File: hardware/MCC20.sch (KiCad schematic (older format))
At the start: 6 parts, among them J101 Conn_01x20, J102 Conn_01x20

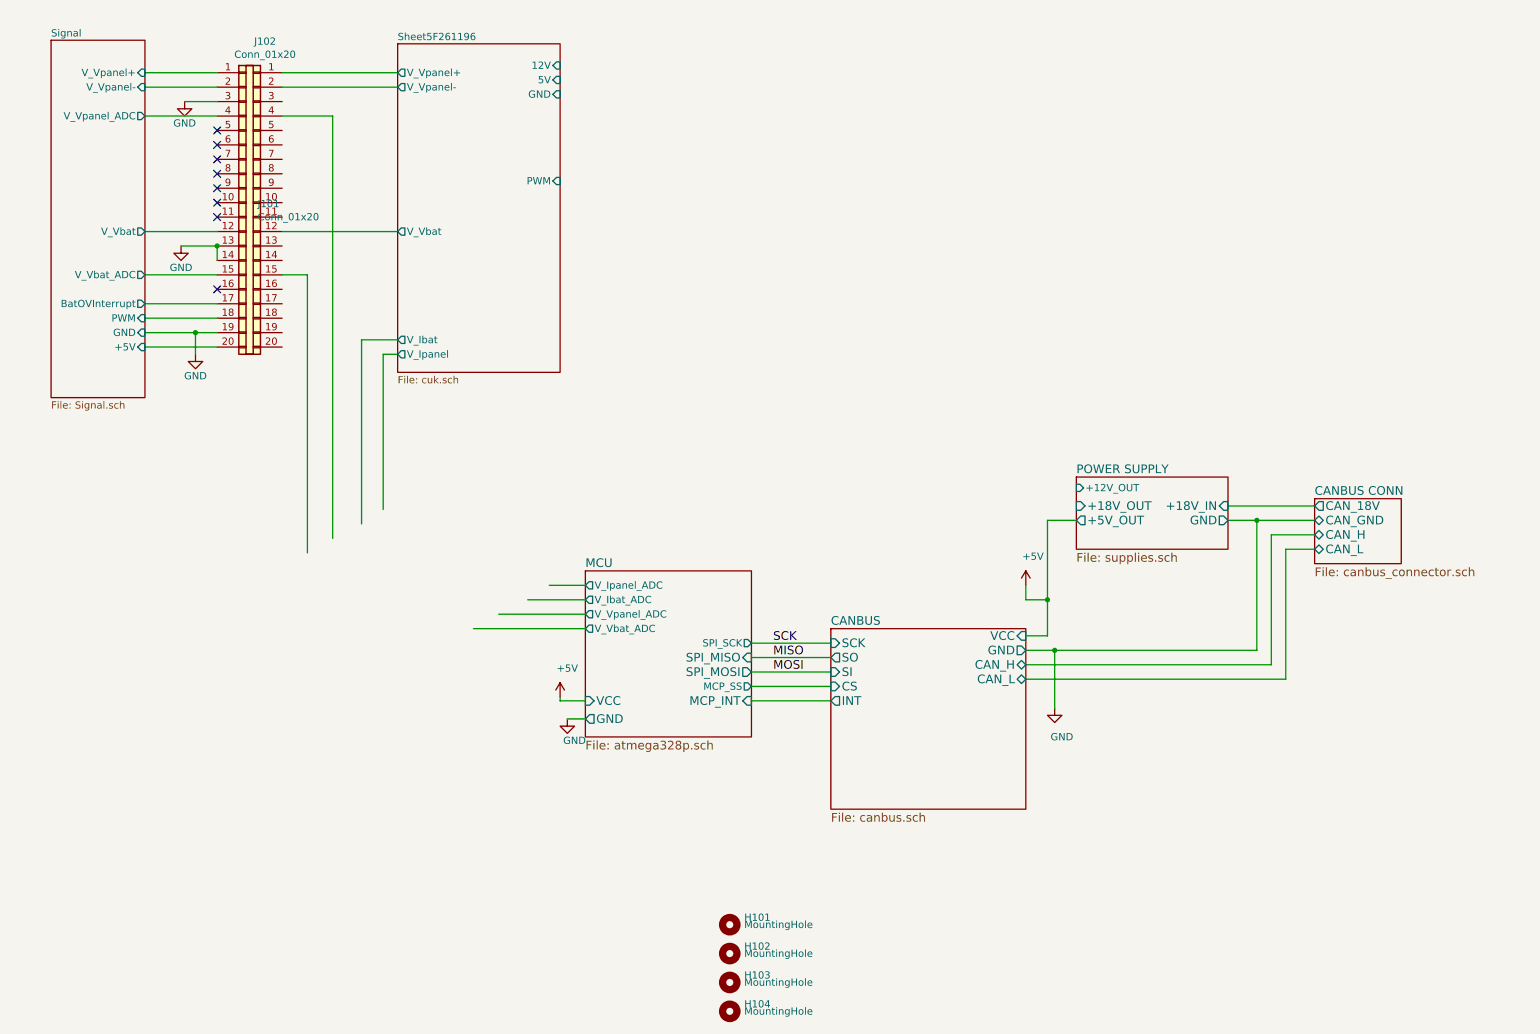
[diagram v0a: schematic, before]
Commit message: schematic and footprint
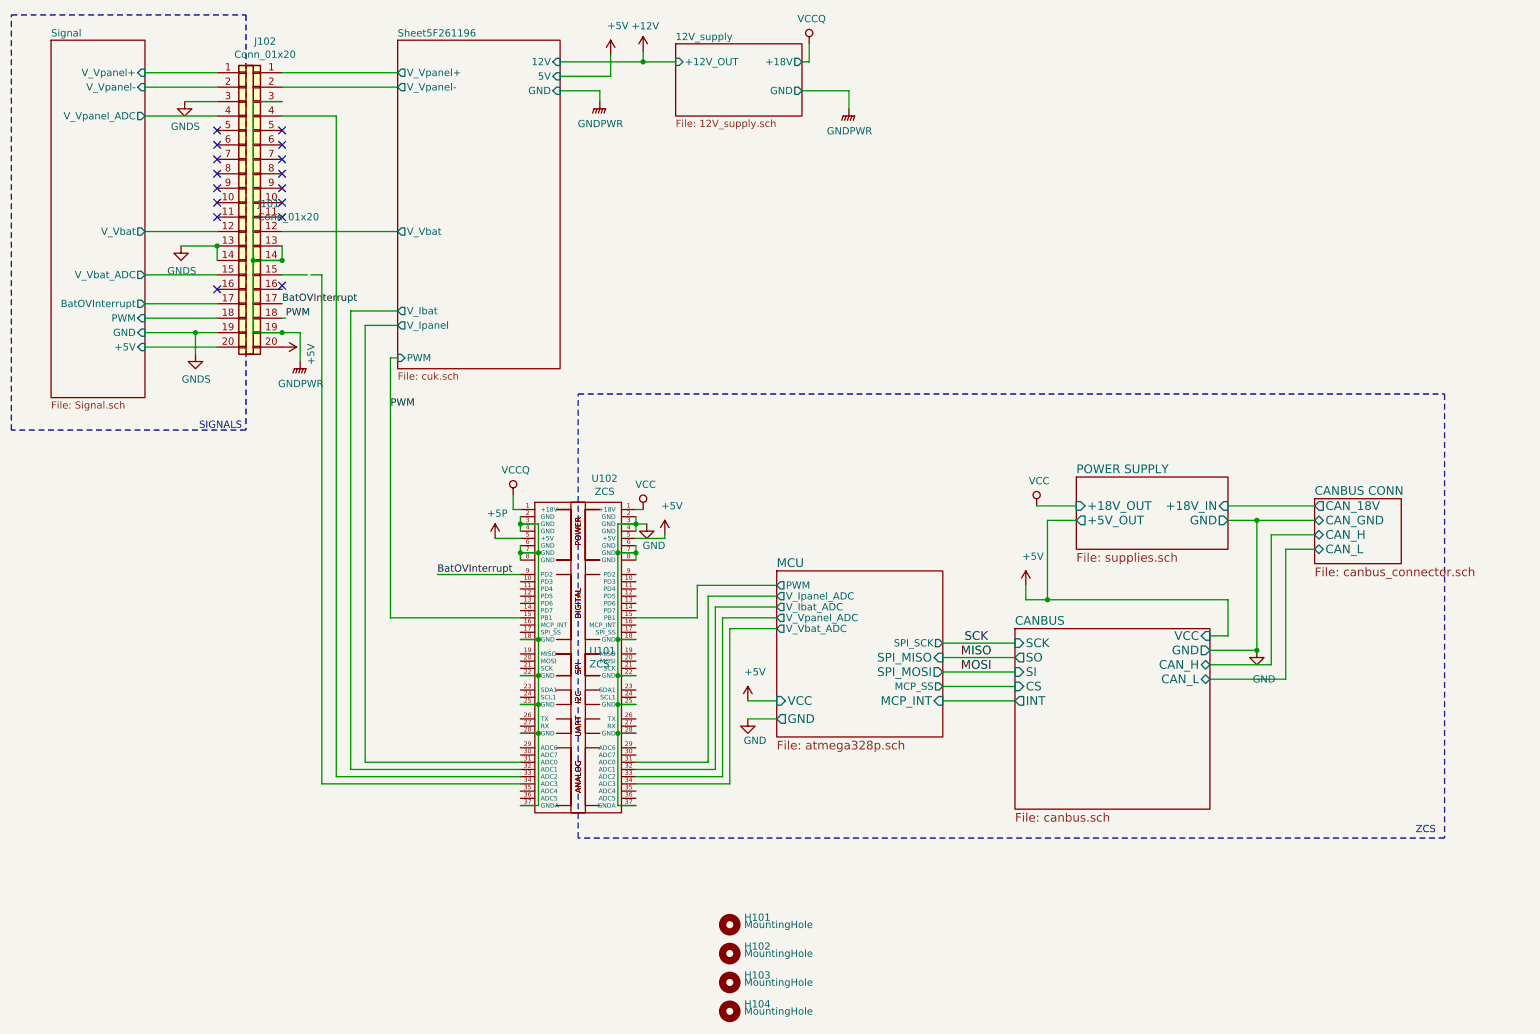
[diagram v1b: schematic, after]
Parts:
- added U101, U102: ZCS, KicadZeniteSolarLibrary18:ZCS18, symbol ZCS:ZCS
- J101: footprint (none) -> Connector_PinHeader_2.54mm:PinHeader_1x20_P2.54mm_Horizontal
- J102: footprint (none) -> Connector_PinSocket_2.54mm:PinSocket_1x20_P2.54mm_Vertical
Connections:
- net labels added: +12V, +5P, BatOVInterrupt, GNDPWR, GNDS, PWM, VCC, VCCQ
- wire segments 56 -> 136
- no-connect marks 8 -> 16
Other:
- note added: "SIGNALS\n"
- note added: "ZCS"
